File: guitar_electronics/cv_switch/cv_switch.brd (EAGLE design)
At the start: 51 x 26.5 mm, 8 parts

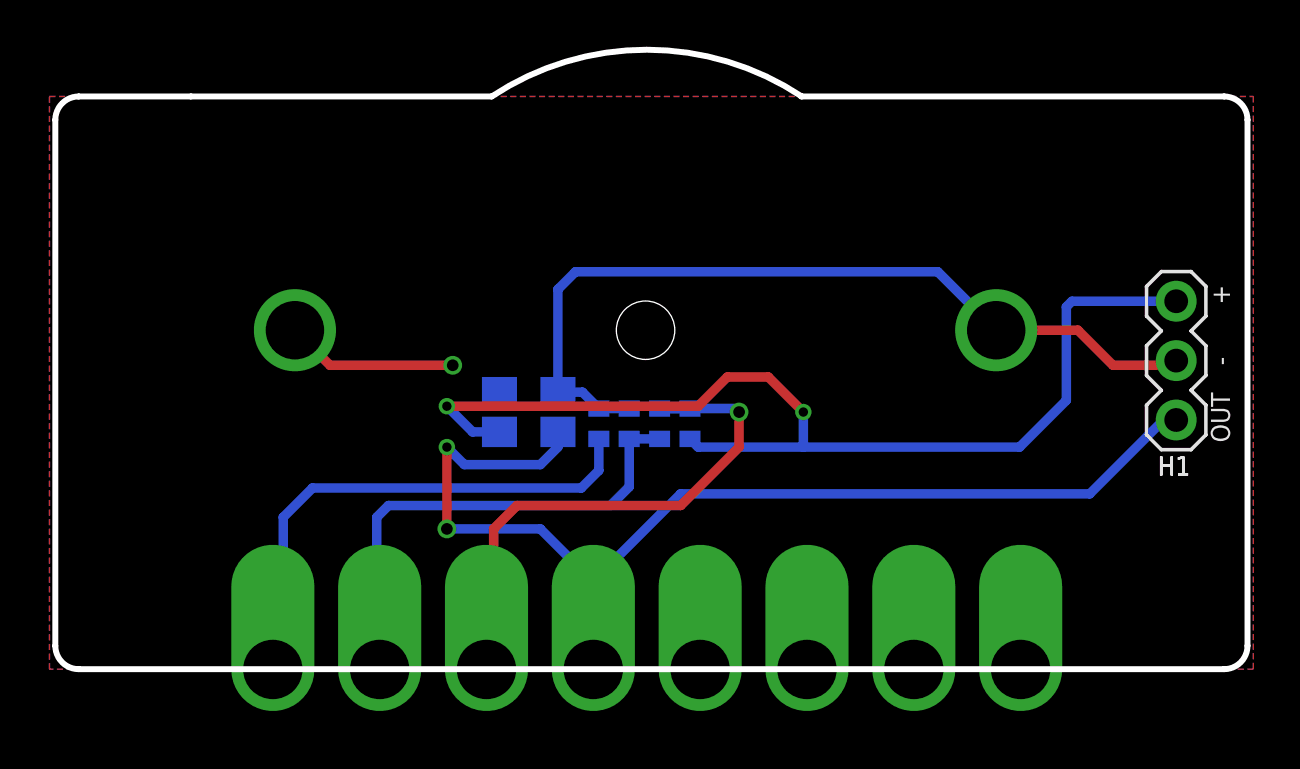
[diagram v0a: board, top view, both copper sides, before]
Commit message: push Nexus peripheral files
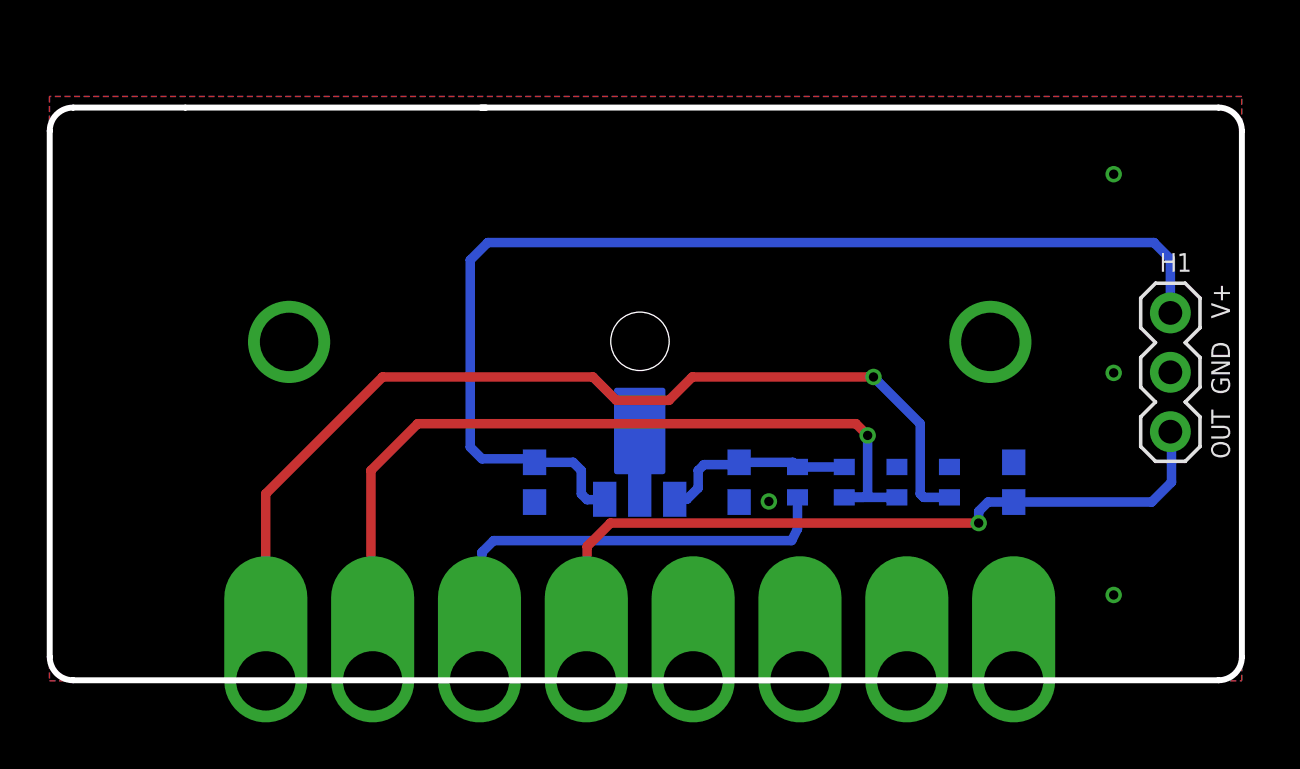
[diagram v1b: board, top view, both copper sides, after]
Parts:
- added C3: 10uF, resistor:C0603
- added U1: CJ75L05, CYCFI_Power:SOT89
- C1, C2: value 10uF -> 1uF; device resistor:C0805 -> resistor:C0603
- R1: value 4.7K -> 1.5K
- R2: value 2.7K -> 3K
- R3: value 2.7K -> 2K
- R4: value 2K -> 1.5K
- moved R4 15.2 mm to (38.5, 8.50)
- moved R3 11.7 mm to (36.2, 8.50)
- moved C2 10.7 mm to (29.5, 8.50), turned to 270 degrees
- moved R2 8.29 mm to (34.0, 8.50)
- moved R1 5.24 mm to (32.0, 8.50), turned to 90 degrees
- moved C1 3.16 mm to (20.8, 8.50), turned to 270 degrees
- moved U$1 0.57 mm to (25.2, 0.00)
- moved H1 0.56 mm to (48.0, 13.2)
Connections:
- removed net N$2: R1.1, R2.2, U$1.N1
- new net +5V: C2.1, R1.2, R2.2, U1.1
- new net N$7: R1.1, U$1.N1
- net GND: now also C3.2, U1.2, U1.2@1
- net N$1: now also C1.1, U1.3; no longer C2.1, R1.2
- net OUT: now also C3.1; no longer C1.1
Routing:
- net GND: track 43.8 -> 0.00 mm, vias 3 -> 6
- net N$2: track 24.4 -> 0.00 mm, vias 1 -> 0
- net N$3: track 22.4 -> 44.0 mm, vias 0 -> 1
- net N$7: track 0.00 -> 20.9 mm
- net N$6: track 21.3 -> 37.1 mm, vias 0 -> 1
- net OUT: track 48.5 -> 34.4 mm, vias 2 -> 1
- net +5V: track 0.00 -> 8.43 mm
- net N$1: track 46.5 -> 48.1 mm, vias 2 -> 0
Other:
- board size 51 x 26.5 mm -> 51 x 24.5 mm
- board text added: "GND"
- board text added: "V+"
- board text added: "v2.5"
- board text removed: "+"
- board text removed: "-"
- board text removed: "C1"
- board text removed: "H1"
- board text removed: "R1"
- board text removed: "R2"
- board text removed: "R3"
- board text removed: "R4"
- board text removed: "v0.97"

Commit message: updated schematic, pcb layout and bom file
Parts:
- R3: value 2K -> 3k
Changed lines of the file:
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@@
 <attribute name="NAME" x="48.86" y="18.299" size="0.8" layer="25" font="vector" ratio="10" rot="R180"/>
 </element>
-<element name="R3" library="resistor" package="R0402" value="2K" x="36.25" y="8.5" smashed="yes" rot="MR270">
+<element name="R3" library="resistor" package="R0402" value="3k" x="36.25" y="8.5" smashed="yes" rot="MR270">
 <attribute name="NAME" x="35.488" y="9.135" size="0.8" layer="26" font="vector" rot="MR270"/>
 <attribute name="VALUE" x="38.282" y="9.135" size="0.8" layer="28" rot="MR270"/>
